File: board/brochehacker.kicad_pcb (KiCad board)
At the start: 2 copper layers, 33 x 33.7 mm, 7 parts, among them IC1 ATTINY85-P, P1 CONN_01X02, SW1 SPST, U1 MAX7219

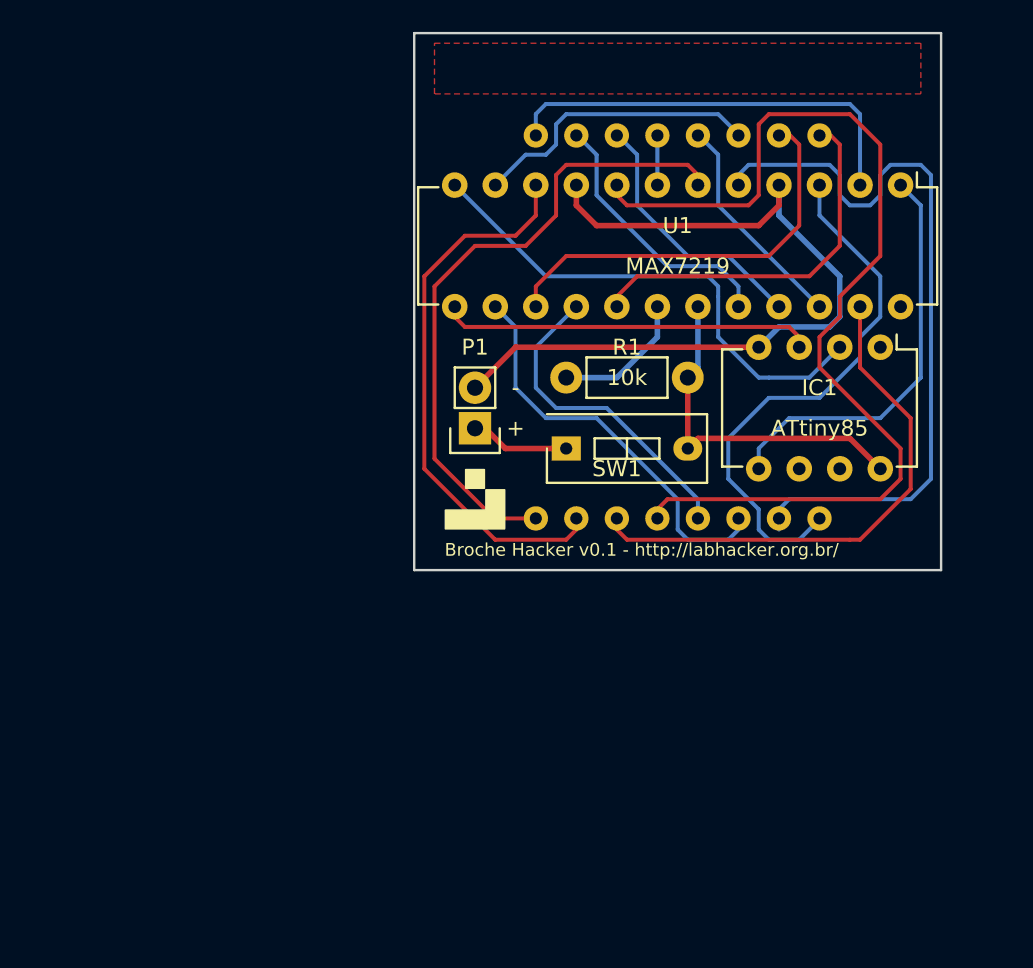
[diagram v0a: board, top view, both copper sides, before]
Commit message: versão camada simples
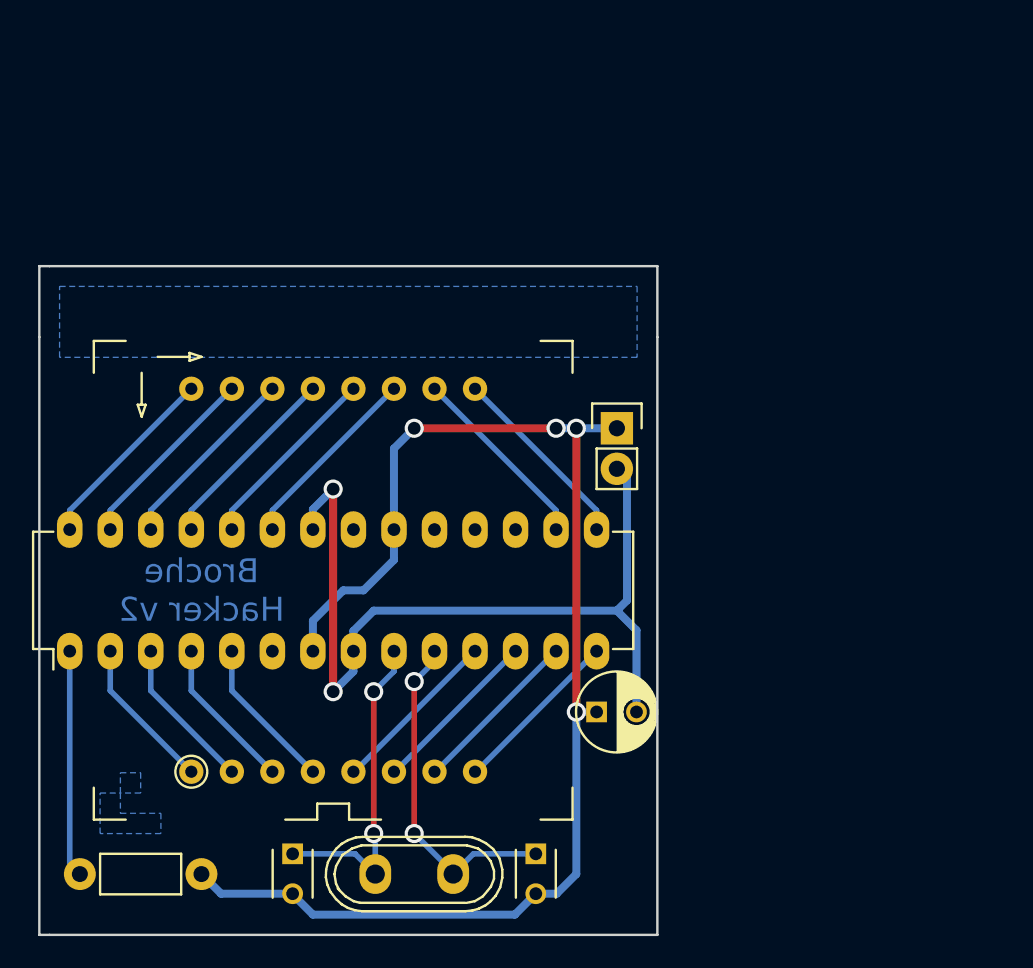
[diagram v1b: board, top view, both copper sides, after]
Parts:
- removed ?: Symbol_OSHW-Logo_SilkScreen, oshw:Symbol_OSHW-Logo_SilkScreen
- removed SW1: SPST, Buttons_Switches_ThroughHole:SW_DIP_x1_Slide
- removed U1: MAX7219, Housings_DIP:DIP-24_W7.62mm
- added C1: 22pF, Capacitors_ThroughHole:C_Disc_D3_P2.5, F.Cu at (175.3, 134.6)
- added C2: 100uF, Capacitors_ThroughHole:C_Radial_D5_L6_P2.5, F.Cu at (179.1, 125.7)
- added C3: 22pF, Capacitors_ThroughHole:C_Disc_D3_P2.5, F.Cu at (160.0, 134.6)
- added Y1: 16MHz, Crystals:Crystal_HC50-U_Vertical, F.Cu at (167.6, 135.9)
- D1: moved to F.Cu
- IC1: value ATTINY85-P -> ATMEGA328-P; footprint Housings_DIP:DIP-8_W7.62mm -> Housings_DIP:DIP-28_W7.62mm_LongPads
- moved IC1 54.3 mm to (146.1, 121.9), turned to 90 degrees
- moved R1 43.6 mm to (154.3, 135.9)
- moved D1 26.8 mm to (162.6, 117.5)
- moved P1 8.89 mm to (180.3, 108.0), turned to 0 degrees
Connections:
- D1 pad 1: /DIG4 -> /ROW5
- D1 pad 10: /SEGC -> /COL4
- D1 pad 11: /SEGE -> /COL6
- D1 pad 12: /DIG3 -> /ROW4
- D1 pad 13: /SEGDP -> /COL1
- D1 pad 14: /DIG1 -> /ROW2
- D1 pad 15: /SEGF -> /COL7
- D1 pad 16: /SEGG -> /COL8
- D1 pad 2: /DIG6 -> /ROW7
- D1 pad 3: /SEGA -> /COL2
- D1 pad 4: /SEGB -> /COL3
- D1 pad 5: /DIG7 -> /ROW8
- D1 pad 6: /SEGD -> /COL5
- D1 pad 7: /DIG5 -> /ROW6
- D1 pad 8: /DIG2 -> /ROW3
- D1 pad 9: /DIG0 -> /ROW1
- IC1 pad 2: Net-(IC1-Pad2) -> /ROW5
- IC1 pad 3: Net-(IC1-Pad3) -> /ROW7
- IC1 pad 4: GND -> /COL2
- IC1 pad 5: Net-(IC1-Pad5) -> /COL3
- IC1 pad 7: Net-(IC1-Pad7) -> VCC
- IC1 pad 8: VCC -> GND
- P1 pad 1: Net-(P1-Pad1) -> VCC
- R1 pad 2: Net-(R1-Pad2) -> Net-(IC1-Pad1)
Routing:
- net /DIG7: track 64.4 -> 0.00 mm
- net VCC: track 22.3 -> 84.9 mm, vias 0 -> 4
- net /DIG6: track 47.5 -> 0.00 mm
- net /DIG2: track 40.7 -> 0.00 mm
- net /DIG5: track 34.9 -> 0.00 mm
- net /DIG4: track 34.5 -> 0.00 mm
- net /SEGD: track 34.1 -> 0.00 mm
- net Net-(IC1-Pad2): track 31.8 -> 0.00 mm
- net /DIG0: track 26.8 -> 0.00 mm
- net /SEGF: track 26.5 -> 0.00 mm
- net Net-(IC1-Pad5): track 25.9 -> 0.00 mm
- net /SEGA: track 25.7 -> 0.00 mm
- net /SEGG: track 25.0 -> 0.00 mm
- net Net-(IC1-Pad3): track 23.4 -> 0.00 mm
- net Net-(C1-Pad1): track 0.00 -> 21.3 mm, vias 0 -> 2
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- added copper zone on B.Cu, net (none)
- removed copper zone on F.Cu, net (none)
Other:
- board size 33 x 33.7 mm -> 38.7 x 41.9 mm
- net class Default: trace_width 0.25 -> 0.35; via_dia 0.6 -> 1.2; via_drill 0.4 -> 0.8
- net class Power: trace_width 0.35 -> 0.5; via_dia 0.6 -> 1.2; via_drill 0.4 -> 0.8
- board text added: "Broche Hacker v2"
- board text removed: "ATtiny85"
- board text removed: "Broche Hacker v0.1 - http://labhacker.org.br/"
- board text removed: "MAX7219"
